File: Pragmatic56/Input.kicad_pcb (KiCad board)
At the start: 2 copper layers, 126.7 x 100.2 mm, 118 parts, among them J1 Conn_02x04_Odd_Even, SW1 SW_Push_45deg, SW10 SW_Push_45deg, SW11 SW_Push_45deg, SW12 SW_Push_45deg, SW13 SW_Push_45deg, SW14 SW_Push_45deg, SW15 SW_Push_45deg, SW16 SW_Push_45deg, SW17 SW_Push_45deg, SW18 SW_Push_45deg, SW19 SW_Push_45deg, SW2 SW_Push_45deg, SW20 SW_Push_45deg, SW21 SW_Push_45deg, SW22 SW_Push_45deg, SW23 SW_Push_45deg, SW24 SW_Push_45deg, SW25 SW_Push_45deg, SW26 SW_Push_45deg, SW27 SW_Push_45deg, SW28 SW_Push_45deg, SW29 SW_Push_45deg, SW3 SW_Push_45deg, SW30 SW_Push_45deg, SW31 SW_Push_45deg, SW32 SW_Push_45deg, SW33 SW_Push_45deg, SW34 SW_Push_45deg, SW35 SW_Push_45deg, SW36 SW_Push_45deg, SW37 SW_Push_45deg, SW38 SW_Push_45deg, SW39 SW_Push_45deg, SW4 SW_Push_45deg, SW40 SW_Push_45deg, SW41 SW_Push_45deg, SW42 SW_Push_45deg, SW43 SW_Push_45deg, SW44 SW_Push_45deg, SW45 SW_Push_45deg, SW46 SW_Push_45deg, SW47 SW_Push_45deg, SW48 SW_Push_45deg, SW5 SW_Push_45deg, SW51 SW_Push_45deg, SW52 SW_Push_45deg, SW53 SW_Push_45deg, SW54 SW_Push_45deg, SW55 SW_Push_45deg, SW56 SW_Push_45deg, SW57 SW_Push_45deg, SW58 SW_Push_45deg, SW6 SW_Push_45deg, SW7 SW_Push_45deg, SW8 SW_Push_45deg, SW9 SW_Push_45deg

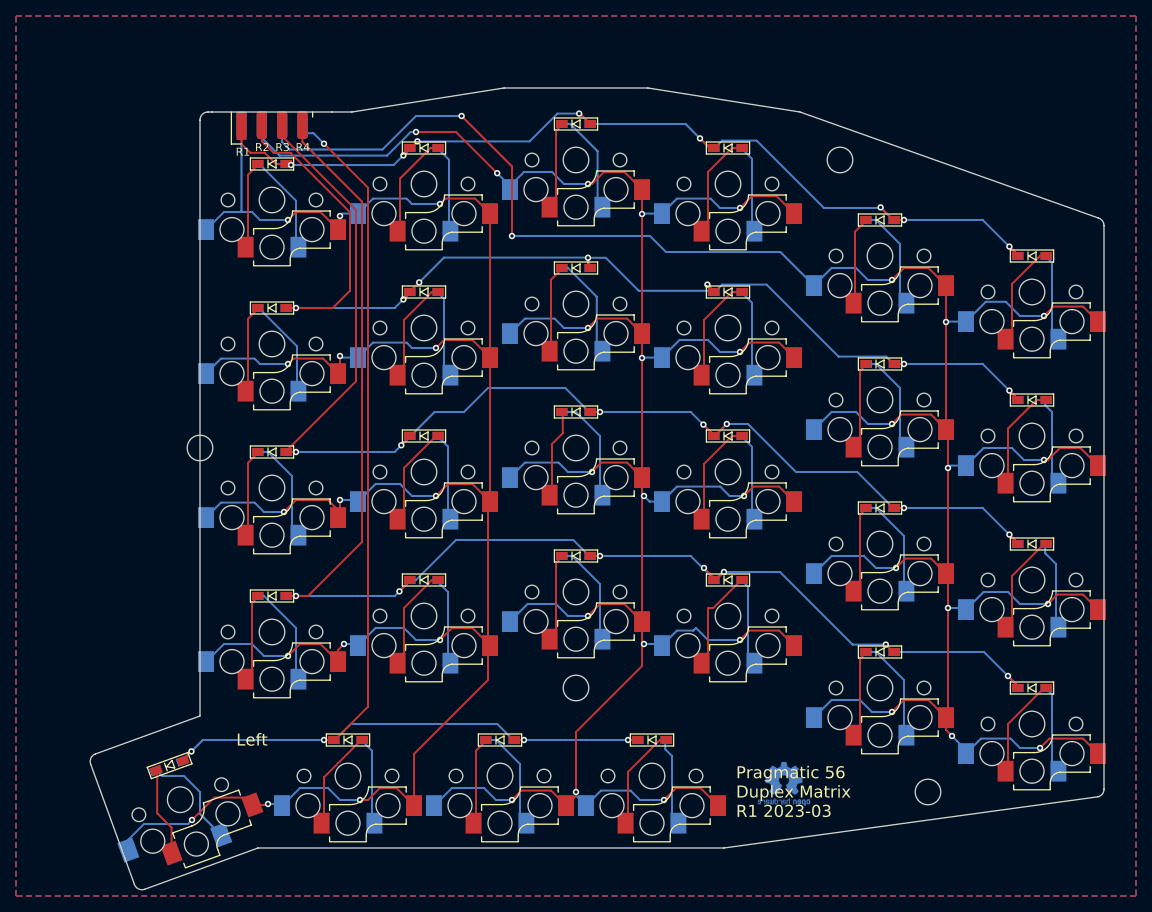
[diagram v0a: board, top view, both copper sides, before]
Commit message: validated
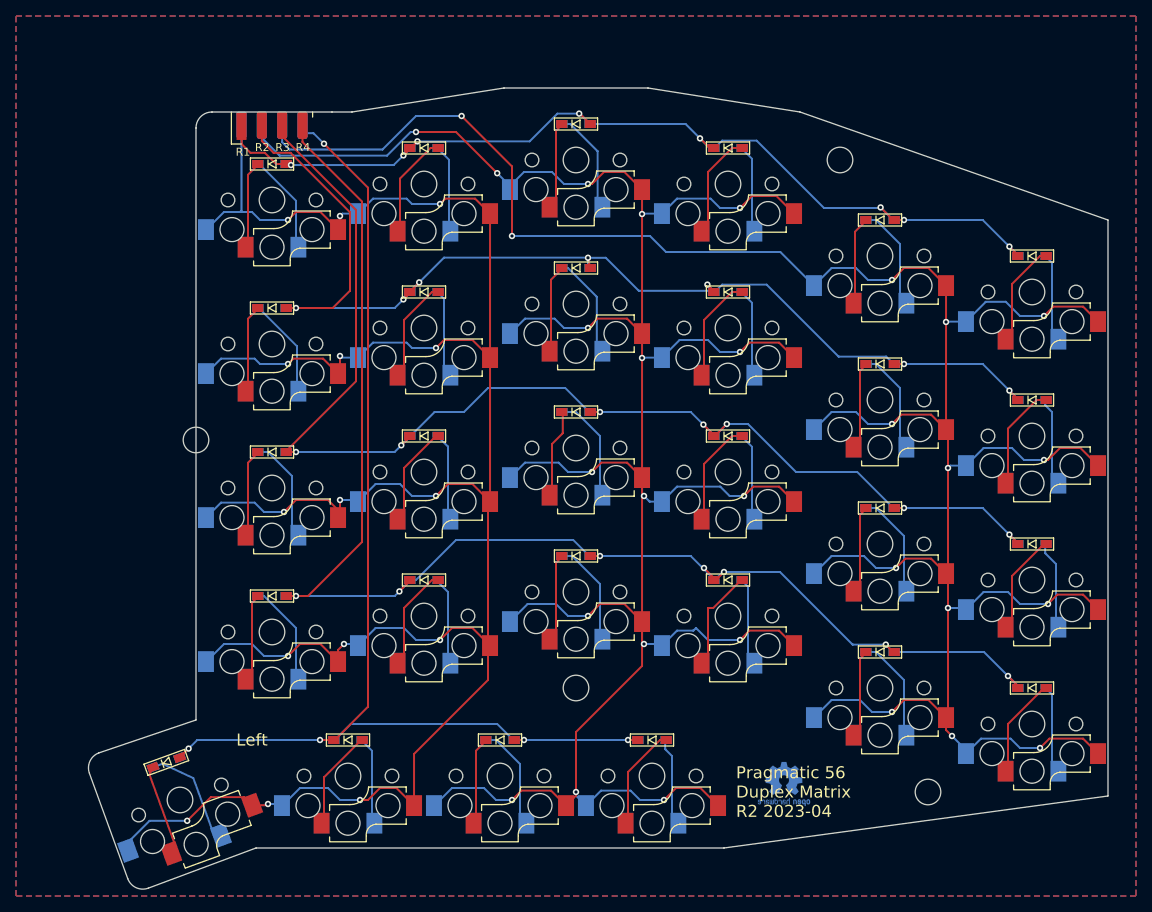
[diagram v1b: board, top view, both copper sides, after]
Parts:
- moved H4 1.12 mm to (120.5, 95.0)
- moved D54 0.57 mm to (116.8, 135.3)
- moved D55 0.55 mm to (116.8, 135.3)
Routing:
- net Row 1: track 121.6 -> 120.5 mm
- net Net-(D21-Pad2): track 13.0 -> 12.0 mm
- net Net-(D9-Pad2): track 13.1 -> 12.3 mm
- net Net-(D55-Pad2): track 13.0 -> 13.7 mm
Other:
- board size 126.7 x 100.2 mm -> 127.4 x 100.1 mm
- board text added: "Pragmatic 56 Duplex Matrix R2 2023-04"
- board text removed: "Pragmatic 56 Duplex Matrix R1 2023-03"
